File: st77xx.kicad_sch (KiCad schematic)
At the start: 8 parts, among them J1 Pins, J2 Flex, Q1 S8050, U1 XC6206PxxxMR

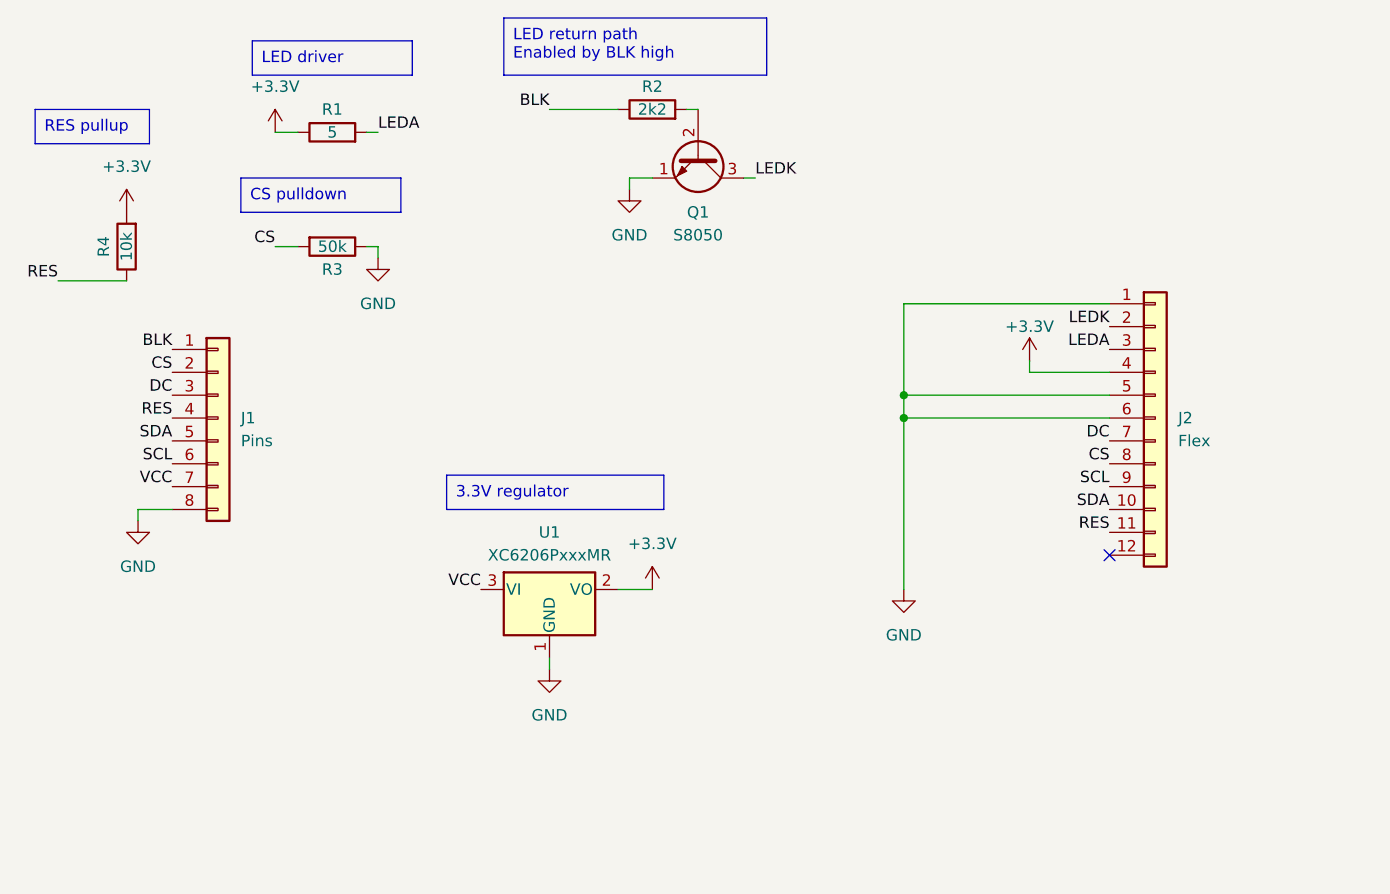
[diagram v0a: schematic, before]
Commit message: Fix schematic
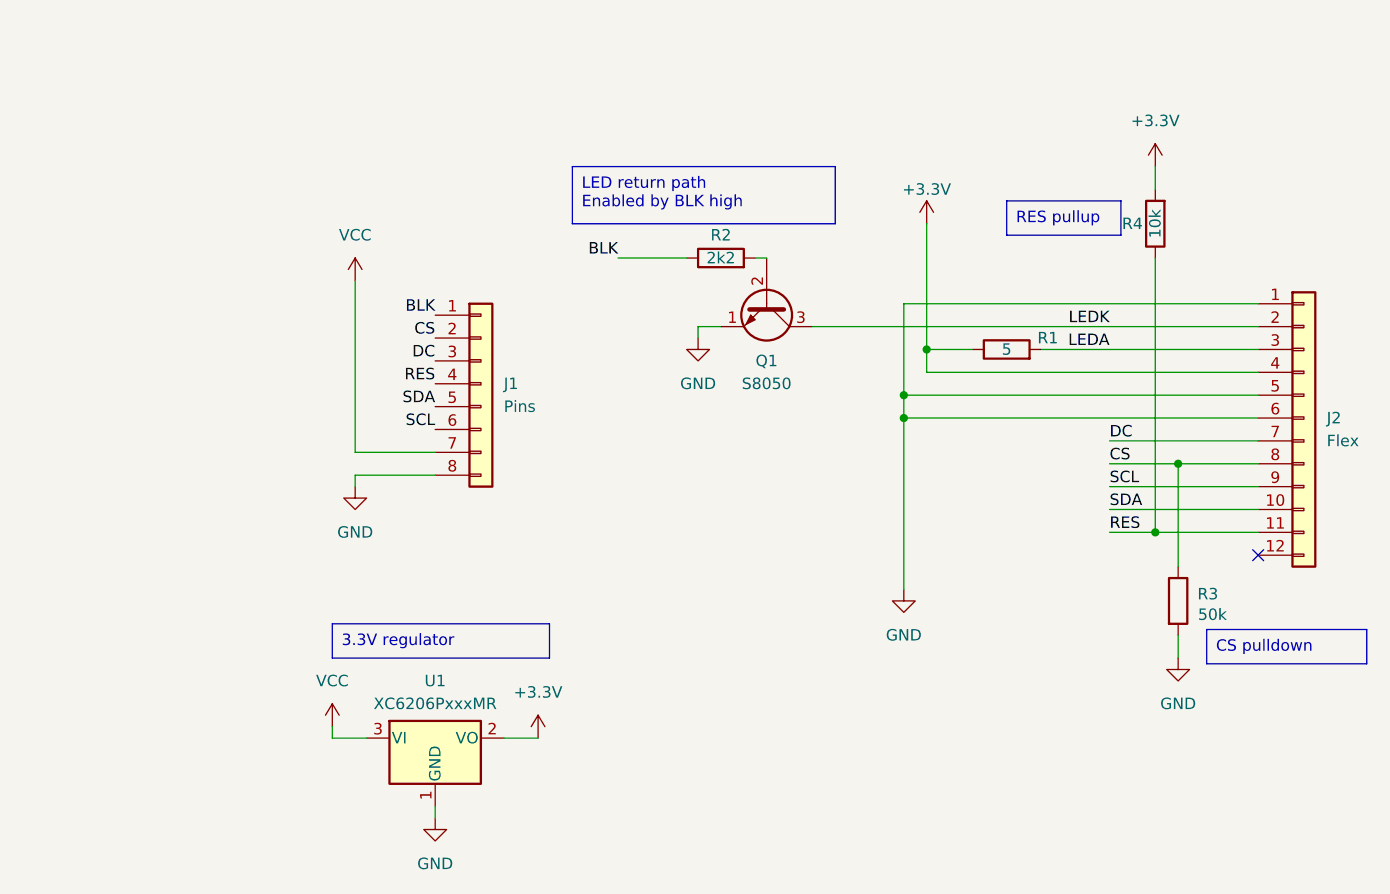
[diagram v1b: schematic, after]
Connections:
- net CS: now also R3.1; no longer R3.2
- net GND: now also R3.2; no longer R3.1
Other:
- moved on the sheet: J1, J2, Q1, R2, U1
